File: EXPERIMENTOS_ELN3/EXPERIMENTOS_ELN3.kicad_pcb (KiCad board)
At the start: 2 copper layers, 100 x 50 mm, 51 parts, among them J1 Screw_Terminal_01x03, J12 MC Out1, J13 MC Out2, J14 Conn_01x07_Socket, J6 MC out

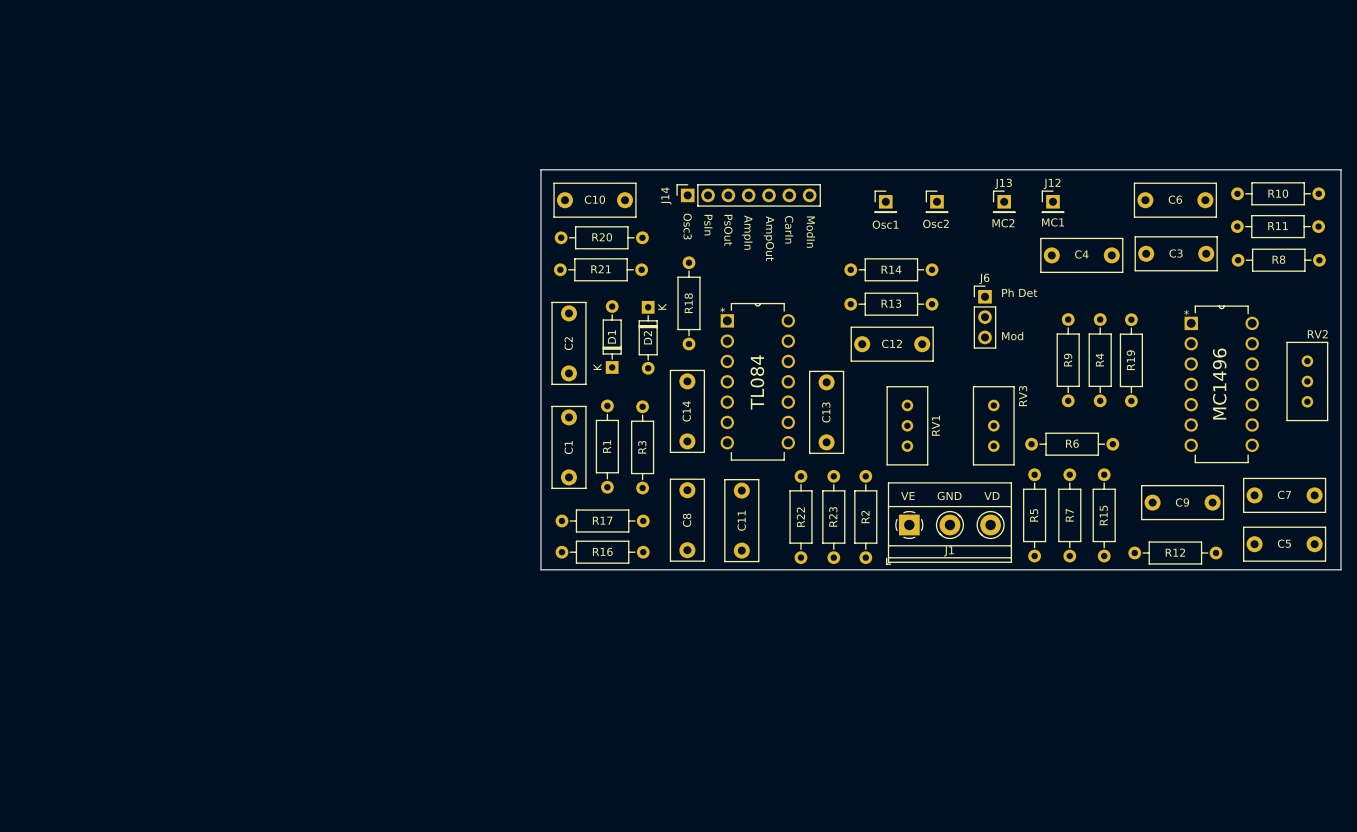
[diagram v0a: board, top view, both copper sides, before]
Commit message: pcb finished
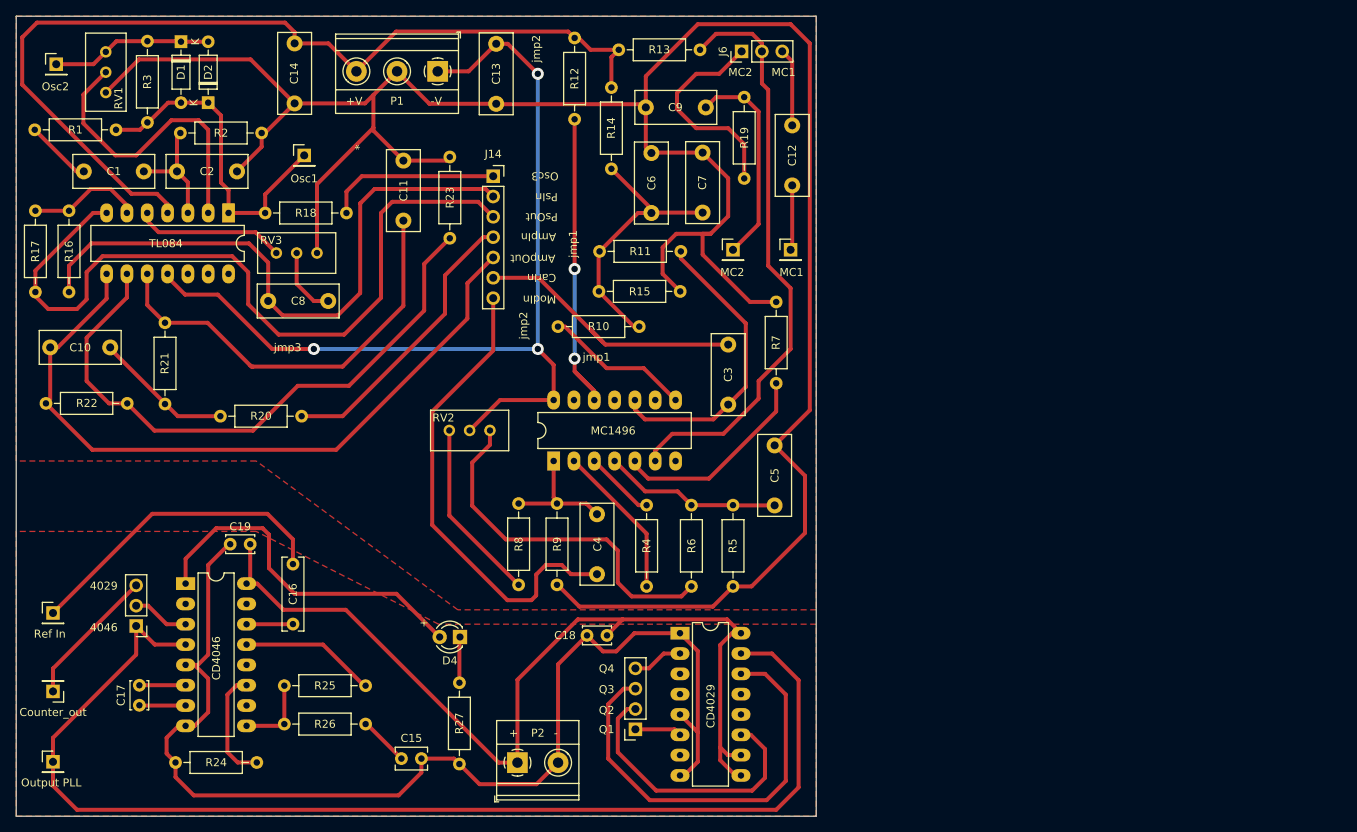
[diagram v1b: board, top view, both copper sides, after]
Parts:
- removed MC1496: MC1496BPG, MC1496BPG:MC1496BPG
- removed TL084: TL084, MC1496BPG:MC1496BPG
- added C15: 68n, Capacitor_THT:C_Disc_D3.8mm_W2.6mm_P2.50mm, F.Cu at (90.5, 140.6)
- added C16: 100n, Capacitor_THT:C_Rect_L9.0mm_W2.5mm_P7.50mm_MKT, F.Cu at (77.0, 116.3)
- added C17: 68n, Capacitor_THT:C_Disc_D3.4mm_W2.1mm_P2.50mm, F.Cu at (57.8, 133.9)
- added C18: 47n, Capacitor_THT:C_Disc_D3.4mm_W2.1mm_P2.50mm, F.Cu at (116.2, 125.2)
- added C19: 47n, Capacitor_THT:C_Disc_D3.4mm_W2.1mm_P2.50mm, F.Cu at (71.7, 113.8)
- added D4: LED, LED_THT:LED_D3.0mm, F.Cu at (97.9, 125.4)
- added J2: F Select, Connector_PinSocket_2.54mm:PinSocket_1x04_P2.54mm_Vertical, F.Cu at (119.8, 136.9)
- added J3: Ref In, Connector_PinHeader_2.54mm:PinHeader_1x01_P2.54mm_Vertical, F.Cu at (47.0, 122.4)
- added J4: F_select_out, Connector_PinHeader_2.54mm:PinHeader_1x01_P2.54mm_Vertical, F.Cu at (47.0, 132.2)
- added J7: Seletor, Connector_PinHeader_2.54mm:PinHeader_1x03_P2.54mm_Vertical, F.Cu at (57.4, 124.0)
- added P1: Screw_Terminal_01x03, TerminalBlock_Phoenix:TerminalBlock_Phoenix_MKDS-1,5-3-5.08_1x03_P5.08mm_Horizontal, F.Cu at (95.1, 54.7)
- added P2: Screw_Terminal_01x02, TerminalBlock_Phoenix:TerminalBlock_Phoenix_MKDS-1,5-2-5.08_1x02_P5.08mm_Horizontal, F.Cu at (105.1, 141.1)
- added R24: 10k, Resistor_THT:R_Axial_DIN0207_L6.3mm_D2.5mm_P10.16mm_Horizontal, F.Cu at (62.3, 141.1)
- added R25: 100k, Resistor_THT:R_Axial_DIN0207_L6.3mm_D2.5mm_P10.16mm_Horizontal, F.Cu at (86.1, 131.5)
- added R26: 4k7, Resistor_THT:R_Axial_DIN0207_L6.3mm_D2.5mm_P10.16mm_Horizontal, F.Cu at (75.9, 136.3)
- added R27: 10k, Resistor_THT:R_Axial_DIN0207_L6.3mm_D2.5mm_P10.16mm_Horizontal, F.Cu at (97.8, 131.1)
- added U1: TL084, Package_DIP:CERDIP-14_W7.62mm_SideBrazed_LongPads, F.Cu at (68.9, 72.4)
- added U2: MC1496, Package_DIP:CERDIP-14_W7.62mm_SideBrazed_LongPads, F.Cu at (109.6, 103.4)
- added U3: 4046, Package_DIP:DIP-16_W7.62mm_LongPads, F.Cu at (63.6, 118.7)
- added U4: 4029, Package_DIP:DIP-16_W7.62mm_LongPads, F.Cu at (125.4, 124.9)
- J1: value Screw_Terminal_01x03 -> Output; footprint TerminalBlock_Phoenix:TerminalBlock_Phoenix_MKDS-1,5-3-5.08_1x03_P5.08mm_Horizontal -> Connector_PinHeader_2.54mm:PinHeader_1x01_P2.54mm_Vertical
- moved Osc2 111.4 mm to (47.4, 53.8)
- moved J1 111.1 mm to (47.0, 141.0)
- moved RV1 109.5 mm to (53.6, 52.3)
- moved R8 108.0 mm to (105.2, 118.9), turned to 90 degrees
- moved RV2 102.2 mm to (101.6, 99.6), turned to 0 degrees
- moved R2 95.8 mm to (62.9, 62.4), turned to 0 degrees
- moved R12 95.1 mm to (112.2, 50.5), turned to -90 degrees
- moved RV3 88.0 mm to (80.0, 77.4), turned to 0 degrees
- moved C7 87.7 mm to (128.2, 64.8), turned to -90 degrees
- moved R22 86.4 mm to (56.3, 96.2), turned to 180 degrees
- moved R1 84.4 mm to (44.7, 62.0), turned to 0 degrees
- moved R11 79.8 mm to (115.3, 77.2)
- moved R3 76.9 mm to (58.8, 50.9)
- moved R10 76.6 mm to (120.3, 86.6), turned to 180 degrees
- moved R17 76.4 mm to (44.8, 72.1), turned to -90 degrees
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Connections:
- J1 pad 1: -12V -> /Experimento5/OUT
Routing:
- net GND: track 0.00 -> 449.5 mm
- net /Experimento5/OUT: track 0.00 -> 149.0 mm
- net -12V: track 0.00 -> 119.6 mm, vias 0 -> 3
- net +12V: track 0.00 -> 118.1 mm
- net VDC: track 0.00 -> 117.2 mm
- net /Phase_shift Out: track 0.00 -> 98.0 mm
- net /Amp Out: track 0.00 -> 90.7 mm
- net /Phase_shift In: track 0.00 -> 77.5 mm
- net Net-(U1C--): track 0.00 -> 76.8 mm
- net Net-(J6-Pin_2): track 0.00 -> 74.5 mm
- net /Sig.In: track 0.00 -> 59.8 mm
- net Net-(J2-Pin_3): track 0.00 -> 53.8 mm
- net Net-(U1C-+): track 0.00 -> 52.9 mm
- net Net-(R6-Pad1): track 0.00 -> 45.3 mm
- net Net-(D4-A): track 0.00 -> 44.5 mm
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- added copper zone on F.Cu, net GND
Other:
- board size 100 x 50 mm -> 100 x 100 mm
- board text added: "+"
- board text added: "+V"
- board text added: "-"
- board text added: "-V"
- board text added: "4029"
- board text added: "4046"
- board text added: "CD4029"
- board text added: "CD4046"
- board text added: "Counter_out"
- board text added: "MC1496"
- board text added: "Output PLL"
- board text added: "Q1"
- board text added: "Q2"
- board text added: "Q3"
- board text added: "Q4"
- board text added: "Ref In"
- board text added: "TL084"
- board text added: "jmp1"
- board text added: "jmp2"
- board text added: "jmp3"
- board text removed: "GND"
- board text removed: "Mod"
- board text removed: "Ph Det"
- board text removed: "VD"
- board text removed: "VE"
